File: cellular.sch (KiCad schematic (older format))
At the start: 55 parts, among them P3 Chip anten, Q1 2SC1815, Q2 2SC1815, Q3 2SC1815, Q4 2SC1815, SW1 SW_PUSH, SW2 SW_PUSH, U1 MP2365DN, U2 SIM800H, U6 SIM HOLD - PPSS-6P

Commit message: add sim800h lib
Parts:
- U2: footprint lib:SIM800H -> (none)
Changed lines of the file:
@@
 LIBS:armory
 LIBS:arduino_shieldsNCL
+LIBS:sim800h
 LIBS:cellular-cache
 EELAYER 26 0
@@
 SIM800L_NETLIGHT
 $Comp
-L +5V #PWR3
+L +5V #PWR1
 U 1 1 57DA6B80
 P 2000 12700
-F 0 "#PWR3" H 2000 12550 50  0001 C CNN
+F 0 "#PWR1" H 2000 12550 50  0001 C CNN
 F 1 "+5V" H 2015 12873 50  0000 C CNN
 F 2 "" H 2000 12700 50  0000 C CNN
@@
 $EndComp
 $Comp
-L GND #PWR18
+L GND #PWR21
 U 1 1 57DA6B94
 P 10000 9400
-F 0 "#PWR18" H 10000 9150 50  0001 C CNN
+F 0 "#PWR21" H 10000 9150 50  0001 C CNN
 F 1 "GND" H 10005 9227 50  0000 C CNN
 F 2 "" H 10000 9400 50  0000 C CNN
@@
 NoConn ~ 2500 13150
 $Comp
-L GND #PWR5
+L GND #PWR10
 U 1 1 57DA6B9E
 P 2300 14450
-F 0 "#PWR5" H 2300 14200 50  0001 C CNN
+F 0 "#PWR10" H 2300 14200 50  0001 C CNN
 F 1 "GND" H 2305 14277 50  0000 C CNN
 F 2 "" H 2300 14450 50  0000 C CNN
@@
 $EndComp
 $Comp
-L VDD #PWR7
+L VDD #PWR12
 U 1 1 57DA6BAA
 P 4950 13090
-F 0 "#PWR7" H 4950 12940 50  0001 C CNN
+F 0 "#PWR12" H 4950 12940 50  0001 C CNN
 F 1 "VDD" H 4967 13263 50  0000 C CNN
 F 2 "" H 4950 13090 50  0000 C CNN
@@
 $EndComp
 $Comp
-L VDD #PWR17
+L VDD #PWR20
 U 1 1 57DA6BAC
 P 10000 8500
-F 0 "#PWR17" H 10000 8350 50  0001 C CNN
+F 0 "#PWR20" H 10000 8350 50  0001 C CNN
 F 1 "VDD" H 10017 8673 50  0000 C CNB
 F 2 "" H 10000 8500 50  0000 C CNN
@@
 NoConn ~ 9200 5150
 $Comp
-L GND #PWR22
+L GND #PWR18
 U 1 1 57DA6BB4
 P 9350 5000
-F 0 "#PWR22" H 9350 4750 50  0001 C CNN
+F 0 "#PWR18" H 9350 4750 50  0001 C CNN
 F 1 "GND" H 9355 4827 50  0000 C CNN
 F 2 "" H 9350 5000 50  0000 C CNN
@@
 NoConn ~ 9050 5525
 $Comp
-L GND #PWR21
+L GND #PWR17
 U 1 1 57DA6BB5
 P 8850 6175
-F 0 "#PWR21" H 8850 5925 50  0001 C CNN
+F 0 "#PWR17" H 8850 5925 50  0001 C CNN
 F 1 "GND" H 8855 6002 50  0000 C CNN
 F 2 "" H 8850 6175 50  0000 C CNN
@@
 $EndComp
 $Comp
-L GND #PWR23
+L GND #PWR19
 U 1 1 57DA6BB8
 P 9510 5560
-F 0 "#PWR23" H 9510 5310 50  0001 C CNN
+F 0 "#PWR19" H 9510 5310 50  0001 C CNN
 F 1 "GND" H 9515 5387 50  0000 C CNN
 F 2 "" H 9510 5560 50  0000 C CNN
@@
 $EndComp
 $Comp
-L SIM800H U2
-U 1 1 58A09BCF
-P 3550 4100
-F 0 "U2" H 3550 6378 50  0000 C CNN
-F 1 "SIM800H" H 3550 6287 50  0000 C CNN
-F 2 "lib:SIM800H" H -16500 -1800 50  0001 C CNN
-F 3 "" H -16500 -1950 60  0000 C CNN
-	1    3550 4100
-	1    0    0    -1
-$EndComp
-$Comp
 L ARDUINO_SHIELD SHIELD1
 U 1 1 58A1A630
@@
 $EndComp
 $Comp
-L GND #PWR2
+L GND #PWR5
 U 1 1 58A2B6B5
 P 2150 9875
-F 0 "#PWR2" H 2150 9625 50  0001 C CNN
+F 0 "#PWR5" H 2150 9625 50  0001 C CNN
 F 1 "GND" H 2155 9702 50  0000 C CNN
 F 2 "" H 2150 9875 50  0000 C CNN
@@
 $EndComp
 $Comp
-L +5V #PWR1
+L +5V #PWR4
 U 1 1 58A2D721
 P 2150 9625
-F 0 "#PWR1" H 2150 9475 50  0001 C CNN
+F 0 "#PWR4" H 2150 9475 50  0001 C CNN
 F 1 "+5V" H 2165 9798 50  0000 C CNN
 F 2 "" H 2150 9625 50  0000 C CNN
@@
 SIM800L_NETLIGHT
 $Comp
-L VCC #PWR4
+L VCC #PWR9
 U 1 1 58A55439
 P 2200 12700
-F 0 "#PWR4" H 2250 12750 50  0001 C CNN
+F 0 "#PWR9" H 2250 12750 50  0001 C CNN
 F 1 "VCC" H 2217 12873 50  0000 C CNN
 F 2 "" H -2300 125 50  0000 C CNN
@@
 $EndComp
 $Comp
-L GND #PWR20
+L GND #PWR23
 U 1 1 58A81DF9
 P 10000 10800
-F 0 "#PWR20" H 10000 10550 50  0001 C CNN
+F 0 "#PWR23" H 10000 10550 50  0001 C CNN
 F 1 "GND" H 10005 10627 50  0000 C CNN
 F 2 "" H 10000 10800 50  0000 C CNN
@@
 $EndComp
 $Comp
-L VDD #PWR19
+L VDD #PWR22
 U 1 1 58A81DFF
 P 10000 9900
-F 0 "#PWR19" H 10000 9750 50  0001 C CNN
+F 0 "#PWR22" H 10000 9750 50  0001 C CNN
 F 1 "VDD" H 10017 10073 50  0000 C CNB
 F 2 "" H 10000 9900 50  0000 C CNN
@@
 $EndComp
 $Comp
-L GND #PWR9
+L GND #PWR3
 U 1 1 58A8A7F7
 P 2150 6350
-F 0 "#PWR9" H 2150 6100 50  0001 C CNN
+F 0 "#PWR3" H 2150 6100 50  0001 C CNN
 F 1 "GND" H 2155 6177 50  0000 C CNN
 F 2 "" H 2150 6350 50  0000 C CNN
@@
 SIM800L_DTR
 $Comp
-L VDD #PWR11
+L VDD #PWR7
 U 1 1 58A999FD
 P 2200 2350
-F 0 "#PWR11" H 2200 2200 50  0001 C CNN
+F 0 "#PWR7" H 2200 2200 50  0001 C CNN
 F 1 "VDD" H 2217 2523 50  0000 C CNN
 F 2 "" H 2200 2350 50  0000 C CNN
@@
 $EndComp
 $Comp
-L GND #PWR12
+L GND #PWR8
 U 1 1 58A9A6B2
 P 2200 5800
-F 0 "#PWR12" H 2200 5550 50  0001 C CNN
+F 0 "#PWR8" H 2200 5550 50  0001 C CNN
 F 1 "GND" H 2205 5627 50  0000 C CNN
 F 2 "" H 2200 5800 50  0000 C CNN
@@
 $EndComp
 $Comp
-L GND #PWR8
+L GND #PWR2
 U 1 1 58AACEEA
 P 2050 2950
-F 0 "#PWR8" H 2050 2700 50  0001 C CNN
+F 0 "#PWR2" H 2050 2700 50  0001 C CNN
 F 1 "GND" H 2055 2777 50  0000 C CNN
 F 2 "" H 2050 2950 50  0000 C CNN
@@
 $EndComp
 $Comp
-L GND #PWR10
+L GND #PWR6
 U 1 1 58ABFCDA
 P 2200 1650
-F 0 "#PWR10" H 2200 1400 50  0001 C CNN
+F 0 "#PWR6" H 2200 1400 50  0001 C CNN
 F 1 "GND" H 2205 1477 50  0000 C CNN
 F 2 "" H 2200 1650 50  0000 C CNN
@@
 NoConn ~ 4250 9950
 $Comp
-L GND #PWR6
+L GND #PWR11
 U 1 1 58AD4688
 P 4350 9200
-F 0 "#PWR6" H 4350 8950 50  0001 C CNN
+F 0 "#PWR11" H 4350 8950 50  0001 C CNN
 F 1 "GND" H 4355 9027 50  0000 C CNN
 F 2 "" H 4350 9200 50  0000 C CNN
@@
 Wire Notes Line
 	6400 3800 10900 3800
+$Comp
+L SIM800H U2
+U 1 1 58A4B172
+P 3550 4100
+F 0 "U2" H 3550 6378 50  0000 C CNN
+F 1 "SIM800H" H 3550 6287 50  0000 C CNN
+F 2 "" H -5050 850 50  0001 C CNN
+F 3 "" H -5050 700 60  0000 C CNN
+	1    3550 4100
+	1    0    0    -1
+$EndComp
 $EndSCHEMATC

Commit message: clean lib
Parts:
- D4: footprint (none) -> lib:do214ac
- SW1, SW2: footprint (none) -> lib:SW_SPST_B3U-1000P-B
- U2: footprint (none) -> lib:SIM800H
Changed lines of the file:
@@
 $EndComp
 $Comp
-L GND #PWR14
+L GND #PWR01
 U 1 1 57DA6B65
 P 7550 14450
-F 0 "#PWR14" H 7550 14200 50  0001 C CNN
+F 0 "#PWR01" H 7550 14200 50  0001 C CNN
 F 1 "GND" H 7555 14277 50  0000 C CNN
 F 2 "" H 7550 14450 50  0000 C CNN
@@
 $EndComp
 $Comp
-L GND #PWR15
+L GND #PWR02
 U 1 1 57DA6B68
 P 7850 9450
-F 0 "#PWR15" H 7850 9200 50  0001 C CNN
+F 0 "#PWR02" H 7850 9200 50  0001 C CNN
 F 1 "GND" H 7855 9277 50  0000 C CNN
 F 2 "" H 7850 9450 50  0000 C CNN
@@
 SIM800L_NETLIGHT
 $Comp
-L +5V #PWR1
+L +5V #PWR03
 U 1 1 57DA6B80
 P 2000 12700
-F 0 "#PWR1" H 2000 12550 50  0001 C CNN
+F 0 "#PWR03" H 2000 12550 50  0001 C CNN
 F 1 "+5V" H 2015 12873 50  0000 C CNN
 F 2 "" H 2000 12700 50  0000 C CNN
@@
 $EndComp
 $Comp
-L GND #PWR21
+L GND #PWR04
 U 1 1 57DA6B94
 P 10000 9400
-F 0 "#PWR21" H 10000 9150 50  0001 C CNN
+F 0 "#PWR04" H 10000 9150 50  0001 C CNN
 F 1 "GND" H 10005 9227 50  0000 C CNN
 F 2 "" H 10000 9400 50  0000 C CNN
@@
 NoConn ~ 2500 13150
 $Comp
-L GND #PWR10
+L GND #PWR05
 U 1 1 57DA6B9E
 P 2300 14450
-F 0 "#PWR10" H 2300 14200 50  0001 C CNN
+F 0 "#PWR05" H 2300 14200 50  0001 C CNN
 F 1 "GND" H 2305 14277 50  0000 C CNN
 F 2 "" H 2300 14450 50  0000 C CNN
@@
 $EndComp
 $Comp
-L VDD #PWR12
+L VDD #PWR06
 U 1 1 57DA6BAA
 P 4950 13090
-F 0 "#PWR12" H 4950 12940 50  0001 C CNN
+F 0 "#PWR06" H 4950 12940 50  0001 C CNN
 F 1 "VDD" H 4967 13263 50  0000 C CNN
 F 2 "" H 4950 13090 50  0000 C CNN
@@
 $EndComp
 $Comp
-L VDD #PWR13
+L VDD #PWR07
 U 1 1 57DA6BAB
 P 7550 14050
-F 0 "#PWR13" H 7550 13900 50  0001 C CNB
+F 0 "#PWR07" H 7550 13900 50  0001 C CNB
 F 1 "VDD" H 7567 14223 50  0000 C CNB
 F 2 "" H 7550 14050 50  0000 C CNN
@@
 $EndComp
 $Comp
-L VDD #PWR20
+L VDD #PWR08
 U 1 1 57DA6BAC
 P 10000 8500
-F 0 "#PWR20" H 10000 8350 50  0001 C CNN
+F 0 "#PWR08" H 10000 8350 50  0001 C CNN
 F 1 "VDD" H 10017 8673 50  0000 C CNB
 F 2 "" H 10000 8500 50  0000 C CNN
@@
 NoConn ~ 9200 5150
 $Comp
-L GND #PWR18
+L GND #PWR09
 U 1 1 57DA6BB4
 P 9350 5000
-F 0 "#PWR18" H 9350 4750 50  0001 C CNN
+F 0 "#PWR09" H 9350 4750 50  0001 C CNN
 F 1 "GND" H 9355 4827 50  0000 C CNN
 F 2 "" H 9350 5000 50  0000 C CNN
@@
 NoConn ~ 9050 5525
 $Comp
-L GND #PWR17
+L GND #PWR010
 U 1 1 57DA6BB5
 P 8850 6175
-F 0 "#PWR17" H 8850 5925 50  0001 C CNN
+F 0 "#PWR010" H 8850 5925 50  0001 C CNN
 F 1 "GND" H 8855 6002 50  0000 C CNN
 F 2 "" H 8850 6175 50  0000 C CNN
@@
 $EndComp
 $Comp
-L GND #PWR19
+L GND #PWR011
 U 1 1 57DA6BB8
 P 9510 5560
-F 0 "#PWR19" H 9510 5310 50  0001 C CNN
+F 0 "#PWR011" H 9510 5310 50  0001 C CNN
 F 1 "GND" H 9515 5387 50  0000 C CNN
 F 2 "" H 9510 5560 50  0000 C CNN
@@
 $EndComp
 $Comp
-L GND #PWR5
+L GND #PWR012
 U 1 1 58A2B6B5
 P 2150 9875
-F 0 "#PWR5" H 2150 9625 50  0001 C CNN
+F 0 "#PWR012" H 2150 9625 50  0001 C CNN
 F 1 "GND" H 2155 9702 50  0000 C CNN
 F 2 "" H 2150 9875 50  0000 C CNN
@@
 $EndComp
 $Comp
-L +5V #PWR4
+L +5V #PWR013
 U 1 1 58A2D721
 P 2150 9625
-F 0 "#PWR4" H 2150 9475 50  0001 C CNN
+F 0 "#PWR013" H 2150 9475 50  0001 C CNN
 F 1 "+5V" H 2165 9798 50  0000 C CNN
 F 2 "" H 2150 9625 50  0000 C CNN
@@
 SIM800L_NETLIGHT
 $Comp
-L VCC #PWR9
+L VCC #PWR014
 U 1 1 58A55439
 P 2200 12700
-F 0 "#PWR9" H 2250 12750 50  0001 C CNN
+F 0 "#PWR014" H 2250 12750 50  0001 C CNN
 F 1 "VCC" H 2217 12873 50  0000 C CNN
 F 2 "" H -2300 125 50  0000 C CNN
@@
 $EndComp
 $Comp
-L PWR_FLAG #FLG1
+L PWR_FLAG #FLG015
 U 1 1 58A554C4
 P 2525 12750
-F 0 "#FLG1" H 2575 12800 50  0001 C CNN
+F 0 "#FLG015" H 2575 12800 50  0001 C CNN
 F 1 "PWR_FLAG" H 2525 12974 50  0000 C CNN
 F 2 "" H -1350 275 50  0000 C CNN
@@
 $EndComp
 $Comp
-L PWR_FLAG #FLG2
+L PWR_FLAG #FLG016
 U 1 1 58A55AC7
 P 4950 14425
-F 0 "#FLG2" H 5000 14475 50  0001 C CNN
+F 0 "#FLG016" H 5000 14475 50  0001 C CNN
 F 1 "PWR_FLAG" H 4950 14648 50  0000 C CNN
 F 2 "" H 875 1525 50  0000 C CNN
@@
 $EndComp
 $Comp
-L GND #PWR23
+L GND #PWR017
 U 1 1 58A81DF9
 P 10000 10800
-F 0 "#PWR23" H 10000 10550 50  0001 C CNN
+F 0 "#PWR017" H 10000 10550 50  0001 C CNN
 F 1 "GND" H 10005 10627 50  0000 C CNN
 F 2 "" H 10000 10800 50  0000 C CNN
@@
 $EndComp
 $Comp
-L VDD #PWR22
+L VDD #PWR018
 U 1 1 58A81DFF
 P 10000 9900
-F 0 "#PWR22" H 10000 9750 50  0001 C CNN
+F 0 "#PWR018" H 10000 9750 50  0001 C CNN
 F 1 "VDD" H 10017 10073 50  0000 C CNB
 F 2 "" H 10000 9900 50  0000 C CNN
@@
 F 0 "SW1" H 2500 6555 50  0000 C CNN
 F 1 "SW_PUSH" H 2500 6464 50  0000 C CNN
-F 2 "" H -6100 -1300 50  0000 C CNN
+F 2 "lib:SW_SPST_B3U-1000P-B" H -6100 -1300 50  0001 C CNN
 F 3 "" H -6100 -1300 50  0000 C CNN
 	1    2500 6300
@@
 $EndComp
 $Comp
-L GND #PWR3
+L GND #PWR019
 U 1 1 58A8A7F7
 P 2150 6350
-F 0 "#PWR3" H 2150 6100 50  0001 C CNN
+F 0 "#PWR019" H 2150 6100 50  0001 C CNN
 F 1 "GND" H 2155 6177 50  0000 C CNN
 F 2 "" H 2150 6350 50  0000 C CNN
@@
 SIM800L_DTR
 $Comp
-L VDD #PWR7
+L VDD #PWR020
 U 1 1 58A999FD
 P 2200 2350
-F 0 "#PWR7" H 2200 2200 50  0001 C CNN
+F 0 "#PWR020" H 2200 2200 50  0001 C CNN
 F 1 "VDD" H 2217 2523 50  0000 C CNN
 F 2 "" H 2200 2350 50  0000 C CNN
@@
 $EndComp
 $Comp
-L GND #PWR8
+L GND #PWR021
 U 1 1 58A9A6B2
 P 2200 5800
-F 0 "#PWR8" H 2200 5550 50  0001 C CNN
+F 0 "#PWR021" H 2200 5550 50  0001 C CNN
 F 1 "GND" H 2205 5627 50  0000 C CNN
 F 2 "" H 2200 5800 50  0000 C CNN
@@
 $EndComp
 $Comp
-L GND #PWR2
+L GND #PWR022
 U 1 1 58AACEEA
 P 2050 2950
-F 0 "#PWR2" H 2050 2700 50  0001 C CNN
+F 0 "#PWR022" H 2050 2700 50  0001 C CNN
 F 1 "GND" H 2055 2777 50  0000 C CNN
 F 2 "" H 2050 2950 50  0000 C CNN
@@
 F 0 "D4" V 3004 1879 50  0000 L CNN
 F 1 "D" V 3095 1879 50  0000 L CNN
-F 2 "" H -6000 -1800 50  0001 C CNN
+F 2 "lib:do214ac" H -6000 -1800 50  0001 C CNN
 F 3 "" H -6000 -1800 50  0001 C CNN
 	1    3050 1800
@@
 F 0 "SW2" H 2550 1855 50  0000 C CNN
 F 1 "SW_PUSH" H 2550 1764 50  0000 C CNN
-F 2 "" H -6050 -6000 50  0000 C CNN
+F 2 "lib:SW_SPST_B3U-1000P-B" H -6050 -6000 50  0001 C CNN
 F 3 "" H -6050 -6000 50  0000 C CNN
 	1    2550 1600
@@
 $EndComp
 $Comp
-L GND #PWR6
+L GND #PWR023
 U 1 1 58ABFCDA
 P 2200 1650
-F 0 "#PWR6" H 2200 1400 50  0001 C CNN
+F 0 "#PWR023" H 2200 1400 50  0001 C CNN
 F 1 "GND" H 2205 1477 50  0000 C CNN
 F 2 "" H 2200 1650 50  0000 C CNN
@@
 $EndComp
 $Comp
-L GND #PWR16
+L GND #PWR024
 U 1 1 58AC7889
 P 7850 10800
-F 0 "#PWR16" H 7850 10550 50  0001 C CNN
+F 0 "#PWR024" H 7850 10550 50  0001 C CNN
 F 1 "GND" H 7855 10627 50  0000 C CNN
 F 2 "" H 7850 10800 50  0000 C CNN
@@
 NoConn ~ 4250 9950
 $Comp
-L GND #PWR11
+L GND #PWR025
 U 1 1 58AD4688
 P 4350 9200
-F 0 "#PWR11" H 4350 8950 50  0001 C CNN
+F 0 "#PWR025" H 4350 8950 50  0001 C CNN
 F 1 "GND" H 4355 9027 50  0000 C CNN
 F 2 "" H 4350 9200 50  0000 C CNN
@@
 F 0 "U2" H 3550 6378 50  0000 C CNN
 F 1 "SIM800H" H 3550 6287 50  0000 C CNN
-F 2 "" H -5050 850 50  0001 C CNN
+F 2 "lib:SIM800H" H -5050 850 50  0001 C CNN
 F 3 "" H -5050 700 60  0000 C CNN
 	1    3550 4100

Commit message: add footprint microsim hold
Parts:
- U6: footprint Wurth_Elektronik_Electromechanic_Input-Output_Connectors_rev16b:693023010811 -> lib:Micro_SIM_6P_PUSH_SKM01
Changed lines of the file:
@@
 LIBS:siliconi
 LIBS:opto
-LIBS:atmel
 LIBS:contrib
 LIBS:valves
-LIBS:ACRONET
 LIBS:LP2985-50DBVR
 LIBS:microsd_socket
@@
 F 0 "U6" V 8235 5375 50  0000 C CNN
 F 1 "SIM HOLD - PPSS-6P" V 8326 5375 50  0000 C CNN
-F 2 "Wurth_Elektronik_Electromechanic_Input-Output_Connectors_rev16b:693023010811" H 8600 5150 60  0001 C CNN
+F 2 "lib:Micro_SIM_6P_PUSH_SKM01" H 8600 5150 60  0001 C CNN
 F 3 "" H 8600 5150 60  0000 C CNN
 	1    8600 5150

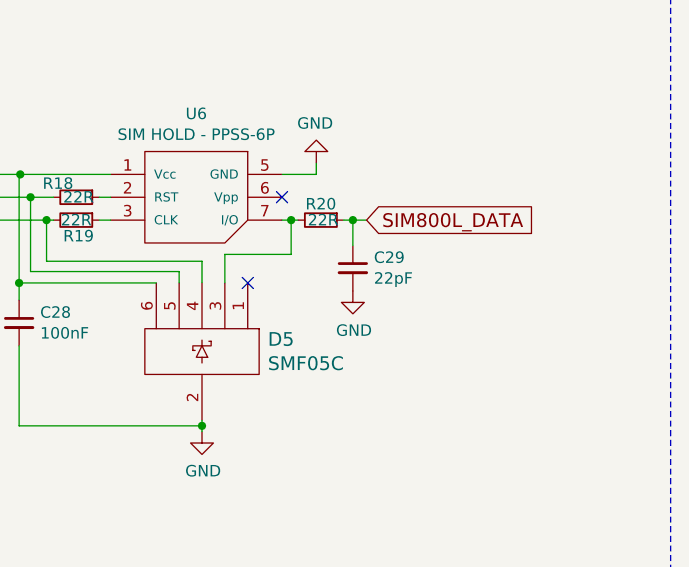
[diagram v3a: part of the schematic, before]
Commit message: change wire connect D5's P3 from low site to high site off R20
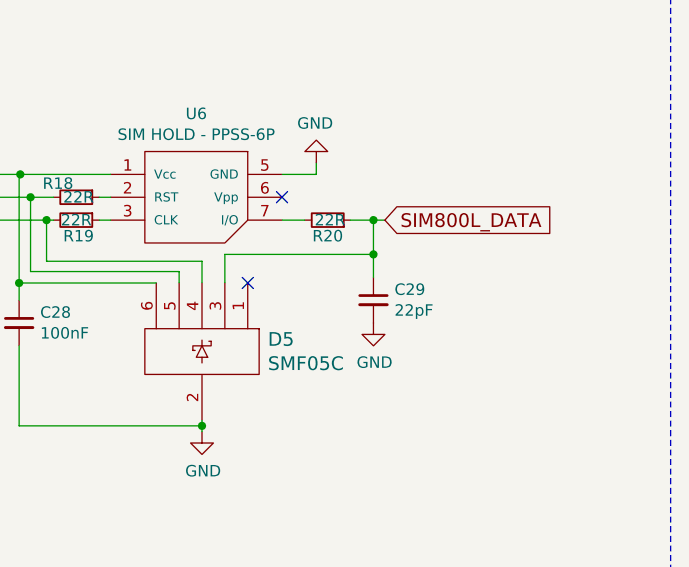
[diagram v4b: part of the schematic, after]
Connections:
- net SIM800L_DATA: now also D5.3
- net at R20.2, U6.7 (I/O): no longer D5.3
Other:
- moved on the sheet: C29, R20
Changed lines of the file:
@@
 	0    1    1    0
 $EndComp
-Text GLabel 9570 5250 2    60   Input ~ 0
+Text GLabel 9650 5250 2    60   Input ~ 0
 SIM800L_DATA
 Text GLabel 7900 5250 0    60   Input ~ 0
@@
 L C_Small C29
 U 1 1 57DA6BB7
-P 9510 5460
-F 0 "C29" H 9602 5506 50  0000 L CNN
-F 1 "22pF" H 9602 5415 50  0000 L CNN
-F 2 "lib:C_0603" H 9510 5460 50  0001 C CNN
-F 3 "" H 9510 5460 50  0000 C CNN
-	1    9510 5460
+P 9600 5600
+F 0 "C29" H 9692 5646 50  0000 L CNN
+F 1 "22pF" H 9692 5555 50  0000 L CNN
+F 2 "lib:C_0603" H 9600 5600 50  0001 C CNN
+F 3 "" H 9600 5600 50  0000 C CNN
+	1    9600 5600
 	1    0    0    -1
 $EndComp
@@
 L GND #PWR011
 U 1 1 57DA6BB8
-P 9510 5560
-F 0 "#PWR011" H 9510 5310 50  0001 C CNN
-F 1 "GND" H 9515 5387 50  0000 C CNN
-F 2 "" H 9510 5560 50  0000 C CNN
-F 3 "" H 9510 5560 50  0000 C CNN
-	1    9510 5560
+P 9600 5700
+F 0 "#PWR011" H 9600 5450 50  0001 C CNN
+F 1 "GND" H 9605 5527 50  0000 C CNN
+F 2 "" H 9600 5700 50  0000 C CNN
+F 3 "" H 9600 5700 50  0000 C CNN
+	1    9600 5700
 	1    0    0    -1
 $EndComp
@@
 L R_Small R20
 U 1 1 57DA6BBA
-P 9370 5250
-F 0 "R20" V 9300 5250 50  0000 C CNN
-F 1 "22R" V 9370 5260 50  0000 C CNN
-F 2 "lib:R_0603" H 9370 5250 50  0001 C CNN
-F 3 "" H 9370 5250 50  0000 C CNN
-	1    9370 5250
-	0    1    1    0
+P 9400 5250
+F 0 "R20" V 9330 5250 50  0000 C CNN
+F 1 "22R" V 9400 5260 50  0000 C CNN
+F 2 "lib:R_0603" H 9400 5250 50  0001 C CNN
+F 3 "" H 9400 5250 50  0000 C CNN
+	1    9400 5250
+	0    1    -1   0
 $EndComp
 $Comp
@@
 $EndComp
 NoConn ~ 4850 4950
+$Comp
+L SIM800H U2
+U 1 1 58A4B172
+P 3550 4100
+F 0 "U2" H 3550 6378 50  0000 C CNN
+F 1 "SIM800H" H 3550 6287 50  0000 C CNN
+F 2 "lib:SIM800H" H -5050 850 50  0001 C CNN
+F 3 "" H -5050 700 60  0000 C CNN
+	1    3550 4100
+	1    0    0    -1
+$EndComp
 Connection ~ 4950 13300
 Connection ~ 4450 14400
@@
 Wire Wire Line
 	8450 5150 8400 5150
-Connection ~ 9240 5250
-Wire Wire Line
-	9240 5400 9240 5250
-Wire Wire Line
-	8950 5400 9240 5400
-Connection ~ 9510 5250
-Wire Wire Line
-	9510 5360 9510 5250
-Wire Wire Line
-	9470 5250 9570 5250
-Wire Wire Line
-	9200 5250 9270 5250
 Wire Wire Line
 	8050 5800 8050 6150
-Wire Wire Line
-	8950 5525 8950 5400
 Wire Wire Line
 	8650 5525 8050 5525
@@
 Wire Notes Line
 	6400 3800 10900 3800
-$Comp
-L SIM800H U2
-U 1 1 58A4B172
-P 3550 4100
-F 0 "U2" H 3550 6378 50  0000 C CNN
-F 1 "SIM800H" H 3550 6287 50  0000 C CNN
-F 2 "lib:SIM800H" H -5050 850 50  0001 C CNN
-F 3 "" H -5050 700 60  0000 C CNN
-	1    3550 4100
-	1    0    0    -1
-$EndComp
+Wire Wire Line
+	9200 5250 9300 5250
+Wire Wire Line
+	8950 5525 8950 5400
+Wire Wire Line
+	9650 5250 9500 5250
+Wire Wire Line
+	9600 5500 9600 5250
+Connection ~ 9600 5250
+Wire Wire Line
+	8950 5400 9600 5400
+Connection ~ 9600 5400
 $EndSCHEMATC
